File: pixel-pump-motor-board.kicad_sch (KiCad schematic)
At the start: 9 parts, among them J2 motor-connector, J3 motor-connector, Q1 STN4NF20L, U1 250X15W104MV4E

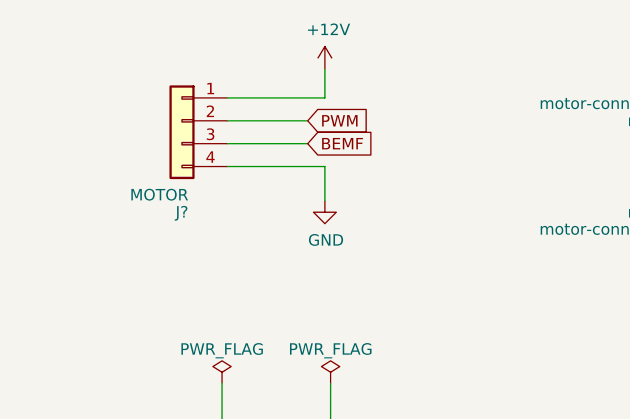
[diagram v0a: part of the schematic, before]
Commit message: Finished
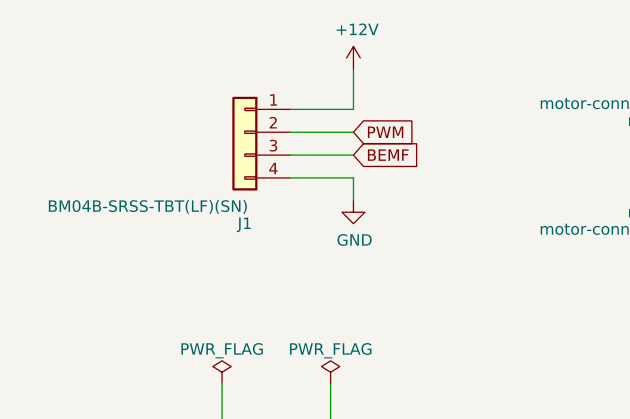
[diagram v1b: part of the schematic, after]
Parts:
- removed J?: MOTOR, Connector_JST:JST_SH_BM04B-SRSS-TB_1x04-1MP_P1.00mm_Vertical, symbol Connector_Generic:Conn_01x04
- added J1: BM04B-SRSS-TBT(LF)(SN), Connector_JST:JST_SH_BM04B-SRSS-TB_1x04-1MP_P1.00mm_Vertical, symbol Connector_Generic:Conn_01x04
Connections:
- net +12V: now also J1.1 (Pin_1)
- net BEMF: now also J1.3 (Pin_3)
- net GND: now also J1.4 (Pin_4)
- net PWM: now also J1.2 (Pin_2)
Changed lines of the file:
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@@
     (stroke (width 0) (type solid) (color 0 0 0 0))
   )
-  (wire (pts (xy 47.625 46.99) (xy 58.42 46.99))
-    (stroke (width 0) (type solid) (color 0 0 0 0))
-  )
-  (wire (pts (xy 47.625 49.53) (xy 56.515 49.53))
-    (stroke (width 0) (type solid) (color 0 0 0 0))
-  )
-  (wire (pts (xy 47.625 52.07) (xy 56.515 52.07))
-    (stroke (width 0) (type solid) (color 0 0 0 0))
-  )
-  (wire (pts (xy 47.625 54.61) (xy 58.42 54.61))
-    (stroke (width 0) (type solid) (color 0 0 0 0))
-  )
-  (wire (pts (xy 58.42 46.99) (xy 58.42 43.815))
-    (stroke (width 0) (type solid) (color 0 0 0 0))
-  )
-  (wire (pts (xy 58.42 54.61) (xy 58.42 58.42))
+  (wire (pts (xy 54.61 48.26) (xy 61.595 48.26))
+    (stroke (width 0) (type solid) (color 0 0 0 0))
+  )
+  (wire (pts (xy 54.61 50.8) (xy 61.595 50.8))
+    (stroke (width 0) (type solid) (color 0 0 0 0))
+  )
+  (wire (pts (xy 54.61 53.34) (xy 61.595 53.34))
+    (stroke (width 0) (type solid) (color 0 0 0 0))
+  )
+  (wire (pts (xy 54.61 55.88) (xy 61.595 55.88))
     (stroke (width 0) (type solid) (color 0 0 0 0))
   )
@@
     (stroke (width 0) (type solid) (color 0 0 0 0))
   )
+  (wire (pts (xy 61.595 48.26) (xy 61.595 43.815))
+    (stroke (width 0) (type solid) (color 0 0 0 0))
+  )
+  (wire (pts (xy 61.595 55.88) (xy 61.595 58.42))
+    (stroke (width 0) (type solid) (color 0 0 0 0))
+  )
   (wire (pts (xy 100.33 49.53) (xy 112.395 49.53))
     (stroke (width 0) (type solid) (color 0 0 0 0))
@@
     (stroke (width 0) (type solid) (color 0 0 0 0))
   )
-  (global_label "PWM" (shape input) (at 56.515 49.53 0)
+  (global_label "PWM" (shape input) (at 61.595 50.8 0)
     (effects (font (size 1.27 1.27)) (justify left))
-    (property "Intersheet References" "${INTERSHEET_REFS}" (id 0) (at 282.575 118.11 0)
-      (effects (font (size 1.27 1.27)) hide)
-    )
-  )
-  (global_label "BEMF" (shape input) (at 56.515 52.07 0)
+    (property "Intersheet References" "${INTERSHEET_REFS}" (id 0) (at 287.655 119.38 0)
+      (effects (font (size 1.27 1.27)) hide)
+    )
+  )
+  (global_label "BEMF" (shape input) (at 61.595 53.34 0)
     (effects (font (size 1.27 1.27)) (justify left))
-    (property "Intersheet References" "${INTERSHEET_REFS}" (id 0) (at 282.575 120.65 0)
-      (effects (font (size 1.27 1.27)) hide)
+    (property "Intersheet References" "${INTERSHEET_REFS}" (id 0) (at 73.2731 53.2606 0)
+      (effects (font (size 1.27 1.27)) (justify left) hide)
     )
   )
@@
     (pin "1")
   )
-  (symbol (lib_id "power:+12V") (at 58.42 43.815 0) (unit 1)
-    (in_bom yes) (on_board yes)
-    (property "Reference" "#PWR01" (id 0) (at 58.42 47.625 0)
-      (effects (font (size 1.27 1.27)) hide)
-    )
-    (property "Value" "+12V" (id 1) (at 58.801 39.4208 0))
-    (property "Footprint" "" (id 2) (at 58.42 43.815 0)
-      (effects (font (size 1.27 1.27)) hide)
-    )
-    (property "Datasheet" "" (id 3) (at 58.42 43.815 0)
+  (symbol (lib_id "power:+12V") (at 61.595 43.815 0) (unit 1)
+    (in_bom yes) (on_board yes)
+    (property "Reference" "#PWR0104" (id 0) (at 61.595 47.625 0)
+      (effects (font (size 1.27 1.27)) hide)
+    )
+    (property "Value" "+12V" (id 1) (at 61.976 39.4208 0))
+    (property "Footprint" "" (id 2) (at 61.595 43.815 0)
+      (effects (font (size 1.27 1.27)) hide)
+    )
+    (property "Datasheet" "" (id 3) (at 61.595 43.815 0)
       (effects (font (size 1.27 1.27)) hide)
     )
@@
     (pin "1")
   )
-  (symbol (lib_id "power:GND") (at 58.42 58.42 0) (unit 1)
-    (in_bom yes) (on_board yes)
-    (property "Reference" "#PWR02" (id 0) (at 58.42 64.77 0)
-      (effects (font (size 1.27 1.27)) hide)
-    )
-    (property "Value" "GND" (id 1) (at 58.547 62.8142 0))
-    (property "Footprint" "" (id 2) (at 58.42 58.42 0)
-      (effects (font (size 1.27 1.27)) hide)
-    )
-    (property "Datasheet" "" (id 3) (at 58.42 58.42 0)
-      (effects (font (size 1.27 1.27)) hide)
-    )
-    (pin "1")
-  )
   (symbol (lib_id "power:GND") (at 59.055 85.09 0) (unit 1)
     (in_bom yes) (on_board yes)
@@
     )
     (property "Datasheet" "" (id 3) (at 59.055 85.09 0)
+      (effects (font (size 1.27 1.27)) hide)
+    )
+    (pin "1")
+  )
+  (symbol (lib_id "power:GND") (at 61.595 58.42 0) (unit 1)
+    (in_bom yes) (on_board yes)
+    (property "Reference" "#PWR0103" (id 0) (at 61.595 64.77 0)
+      (effects (font (size 1.27 1.27)) hide)
+    )
+    (property "Value" "GND" (id 1) (at 61.722 62.8142 0))
+    (property "Footprint" "" (id 2) (at 61.595 58.42 0)
+      (effects (font (size 1.27 1.27)) hide)
+    )
+    (property "Datasheet" "" (id 3) (at 61.595 58.42 0)
       (effects (font (size 1.27 1.27)) hide)
     )
@@
     (pin "2")
   )
-  (symbol (lib_id "Connector_Generic:Conn_01x04") (at 42.545 49.53 0) (mirror y) (unit 1)
-    (in_bom yes) (on_board yes)
-    (property "Reference" "J?" (id 0) (at 42.545 59.69 0))
-    (property "Value" "MOTOR" (id 1) (at 40.005 57.785 0))
-    (property "Footprint" "Connector_JST:JST_SH_BM04B-SRSS-TB_1x04-1MP_P1.00mm_Vertical" (id 2) (at 42.545 49.53 0)
-      (effects (font (size 1.27 1.27)) hide)
-    )
-    (property "Datasheet" "~" (id 3) (at 42.545 49.53 0)
-      (effects (font (size 1.27 1.27)) hide)
-    )
-    (property "Source" "https://lcsc.com/product-detail/Wire-To-Board-Wire-To-Wire-Connector_BOOMELE-Boom-Precision-Elec-C145961_C145961.html" (id 4) (at 42.545 49.53 0)
+  (symbol (lib_id "Connector_Generic:Conn_01x04") (at 49.53 50.8 0) (mirror y) (unit 1)
+    (in_bom yes) (on_board yes)
+    (property "Reference" "J1" (id 0) (at 49.53 60.96 0))
+    (property "Value" "BM04B-SRSS-TBT(LF)(SN)" (id 1) (at 38.735 59.055 0))
+    (property "Footprint" "Connector_JST:JST_SH_BM04B-SRSS-TB_1x04-1MP_P1.00mm_Vertical" (id 2) (at 49.53 50.8 0)
+      (effects (font (size 1.27 1.27)) hide)
+    )
+    (property "Datasheet" "~" (id 3) (at 49.53 50.8 0)
+      (effects (font (size 1.27 1.27)) hide)
+    )
+    (property "Source" "https://lcsc.com/product-detail/Wire-To-Board-Wire-To-Wire-Connector_BOOMELE-Boom-Precision-Elec-C145961_C145961.html" (id 4) (at 49.53 50.8 0)
       (effects (font (size 1.27 1.27)) hide)
     )
@@
       (reference "#FLG0102") (unit 1) (value "PWR_FLAG") (footprint "")
     )
-    (path "/7c1f7596-2adc-4ddd-81b2-8364f9dd10e7"
-      (reference "#PWR01") (unit 1) (value "+12V") (footprint "")
-    )
-    (path "/fe4571d6-4bac-4c5e-995d-3b824025cf76"
-      (reference "#PWR02") (unit 1) (value "GND") (footprint "")
-    )
     (path "/0bd113ac-c401-4364-b116-e3829096fe8c"
       (reference "#PWR03") (unit 1) (value "+12V") (footprint "")
@@
       (reference "#PWR0102") (unit 1) (value "GND") (footprint "")
     )
+    (path "/0777afb6-c9f5-40d3-a69c-cf76b40a7a2d"
+      (reference "#PWR0103") (unit 1) (value "GND") (footprint "")
+    )
+    (path "/bd142016-c6ea-444a-843a-17a19fa62852"
+      (reference "#PWR0104") (unit 1) (value "+12V") (footprint "")
+    )
     (path "/1f7a19e5-e285-4bb1-bf4e-7d1ea9a40a35"
       (reference "C1") (unit 1) (value "C_Polarized") (footprint "Capacitor_Tantalum_SMD:CP_EIA-3216-18_Kemet-A")
@@
       (reference "D1") (unit 1) (value "SOD4007") (footprint "Diode_SMD:D_SOD-123F")
     )
+    (path "/80f92d9a-5f30-4aa7-abbe-2a03b44d3c62"
+      (reference "J1") (unit 1) (value "BM04B-SRSS-TBT(LF)(SN)") (footprint "Connector_JST:JST_SH_BM04B-SRSS-TB_1x04-1MP_P1.00mm_Vertical")
+    )
     (path "/d44ad972-8a51-43a4-b571-d28629d63fde"
       (reference "J2") (unit 1) (value "motor-connector") (footprint "motor-mount:motor-mount")
@@
       (reference "J3") (unit 1) (value "motor-connector") (footprint "motor-mount:motor-mount")
     )
-    (path "/d396a52b-e83f-4e49-aa4f-d1d81b7134a9"
-      (reference "J?") (unit 1) (value "MOTOR") (footprint "Connector_JST:JST_SH_BM04B-SRSS-TB_1x04-1MP_P1.00mm_Vertical")
-    )
     (path "/027211cc-9745-45fd-aa4e-2bf54759e7b3"
